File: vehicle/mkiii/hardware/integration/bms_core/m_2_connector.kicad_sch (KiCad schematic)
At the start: 1 part, among them J5 J_PCIe_x1

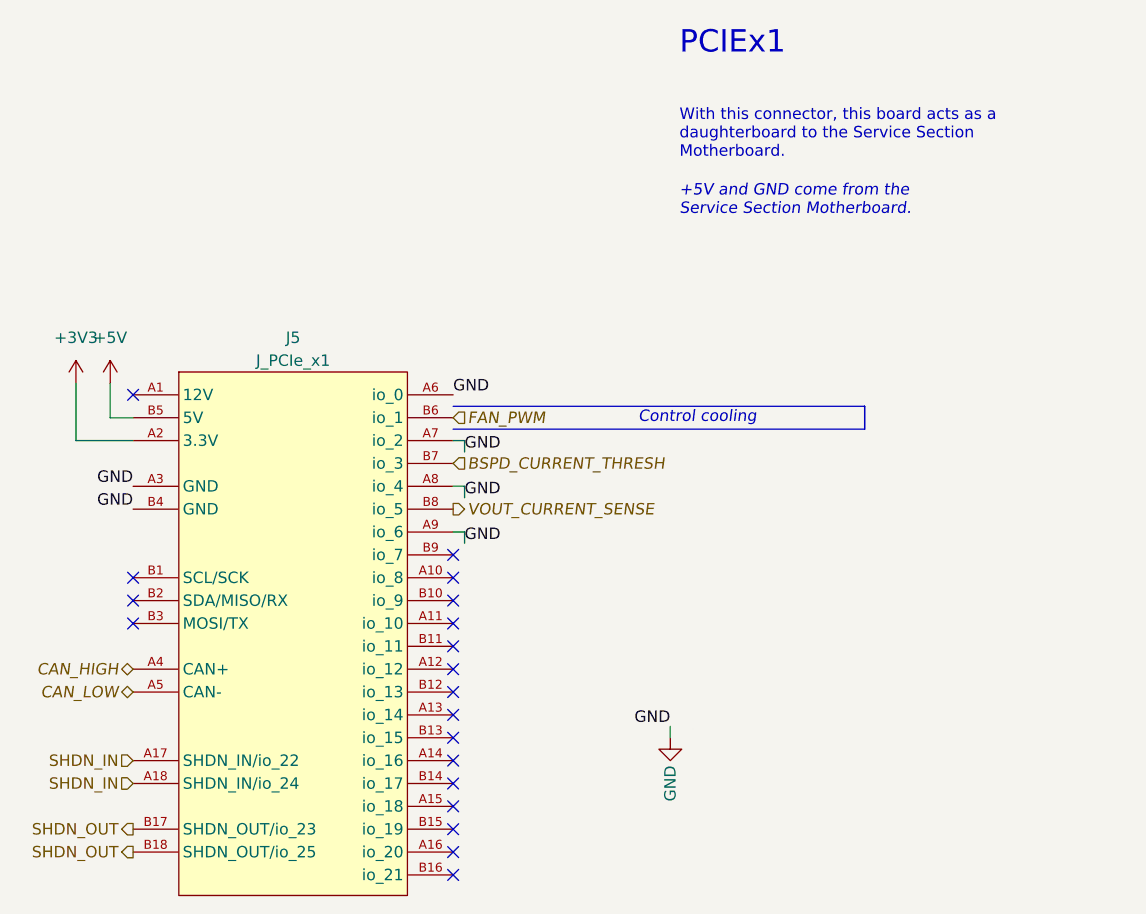
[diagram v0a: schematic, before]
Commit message: Changes according to feedback
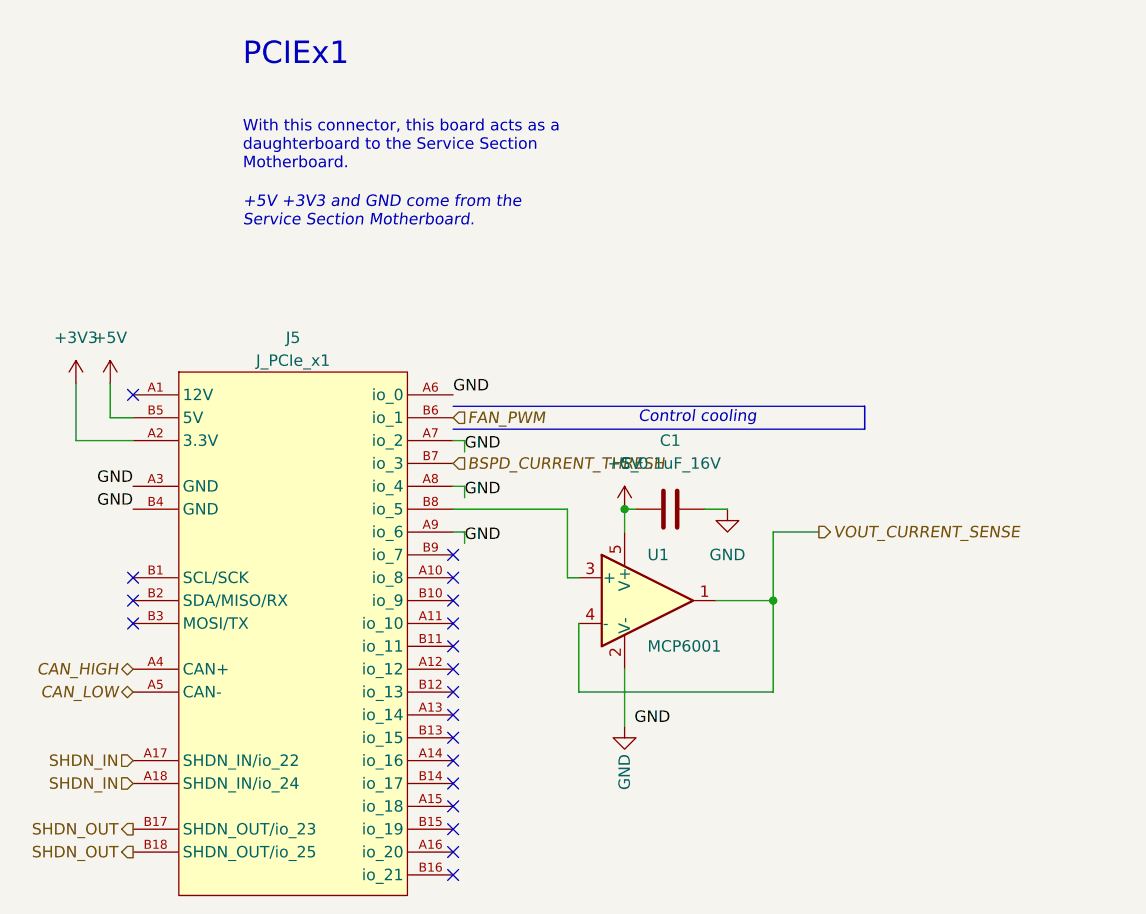
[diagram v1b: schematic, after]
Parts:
- added C1: C_0.1uF_16V, OEM:C_0603_1608Metric, symbol OEM:C_0.1uF_16V_0603
- added U1: MCP6001, Package_TO_SOT_SMD:SOT-353_SC-70-5, symbol OEM:MCP6001
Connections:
- net +5V: now also C1.2, U1.5 (V+)
- net GND: now also C1.1, U1.2 (V-)
- net VOUT_CURRENT_SENSE: now also U1.1, U1.4 (-); no longer J5.B8 (io_5)
- new net: J5.B8 (io_5), U1.3 (+)
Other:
- note added: "+5V +3V3 and GND come from the Service Section Motherboard."
- note removed: "+5V and GND come from the Service Section Motherboard."
